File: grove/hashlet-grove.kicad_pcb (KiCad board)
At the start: 2 copper layers, 20 x 20 mm, 5 parts, among them P1 TWIG_2.0, U1 ATSHA204A

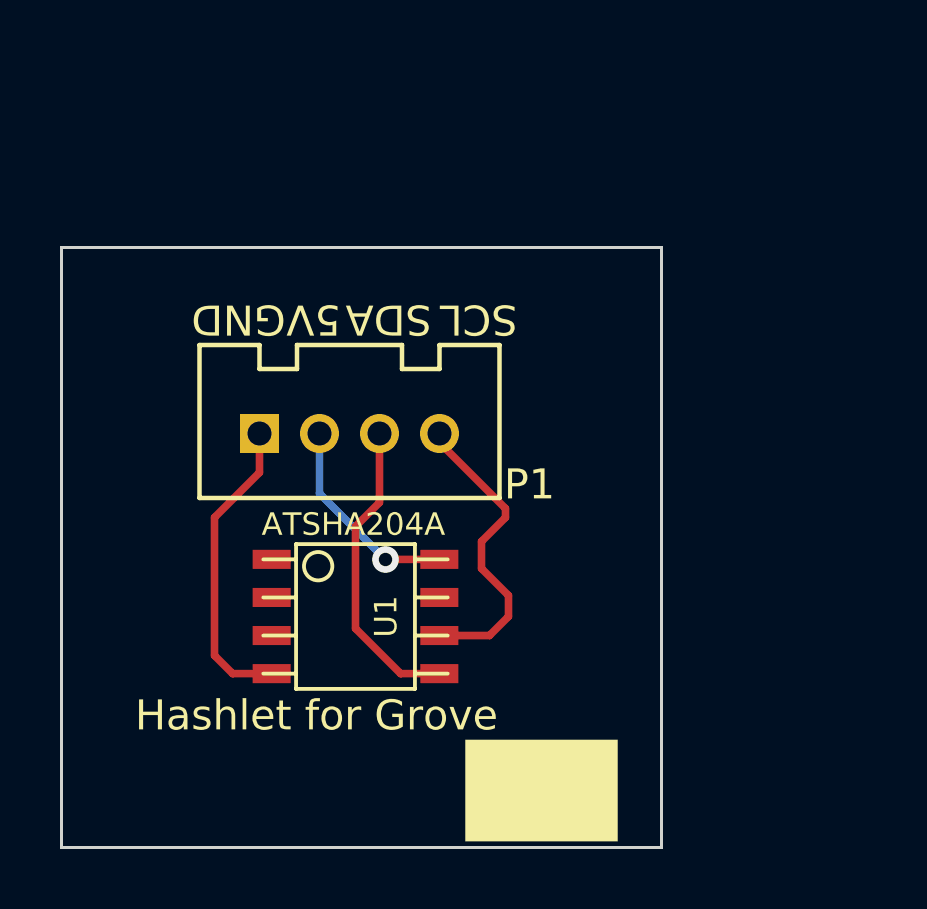
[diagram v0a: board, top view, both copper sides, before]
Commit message: Hashlet for Grove rev v1
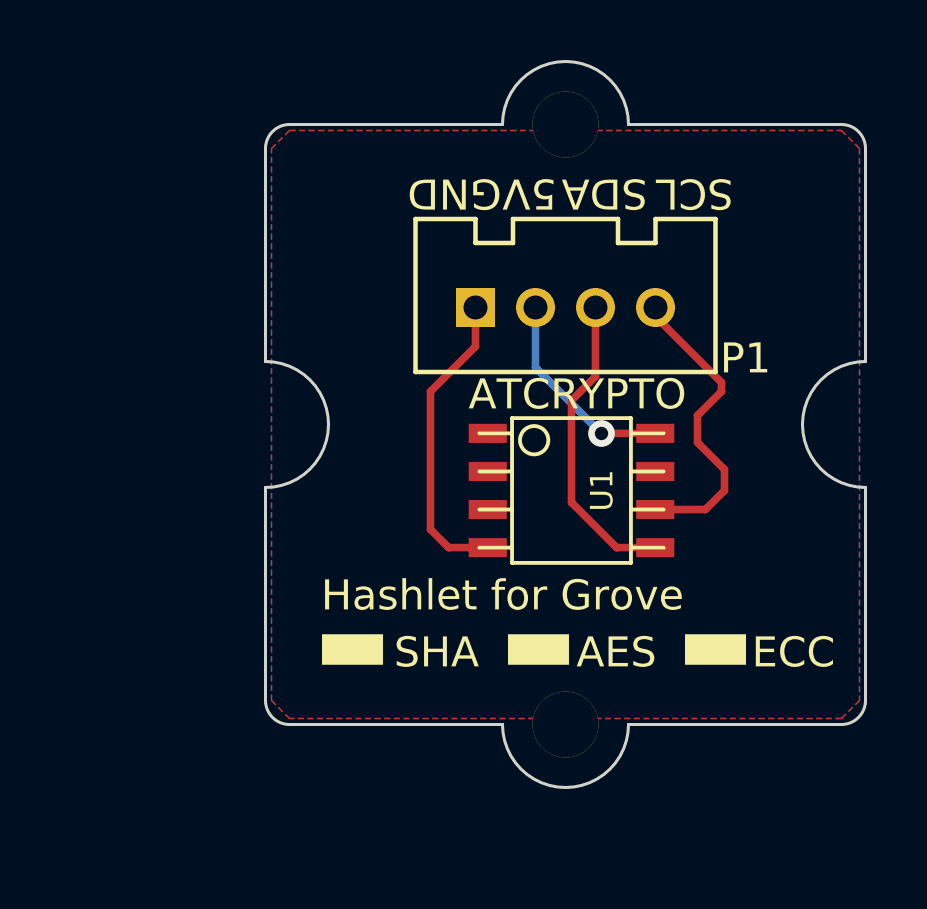
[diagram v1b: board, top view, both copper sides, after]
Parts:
- added G***: CHIPPAD, CHIPPAD, F.Cu at (202.9, 147.5)
- added G***: CHIPPAD, CHIPPAD, F.Cu at (209.1, 147.5)
- added G***: CHIPPAD, CHIPPAD, F.Cu at (215.0, 147.5)
- added HoleA: P***, 1pin, F.Cu at (210.0, 130.0)
- added HoleB: P***, 1pin, F.Cu at (210.0, 150.0)
- G***: moved to B.Cu
- U1: value ATSHA204A -> ATCRYPTO
- moved G*** 22.3 mm to (216.3, 133.2)
- moved G*** 8.67 mm to (215.9, 146.7)
- moved P1 8.34 mm to (210.0, 136.1)
- moved U1 8.34 mm to (210.2, 142.2)
- moved G*** 5.69 mm to (211.4, 141.4)
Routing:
- added copper zone on B.Cu, net GND
- added copper zone on F.Cu, net GND
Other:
- board size 20 x 20 mm -> 20 x 24.2 mm
- board text added: "AES"
- board text added: "ECC"
- board text added: "Module ID"
- board text added: "SHA"
- board text added: "moonpunch.org"
